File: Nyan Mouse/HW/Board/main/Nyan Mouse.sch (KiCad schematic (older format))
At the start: 11 parts, among them M101 BATTBALANCE-2S, P101 CONN_20X2, P102 CONN_4, P103 CONN_2, P104 CONN_2, U101 DRV8837, U102 DRV8837

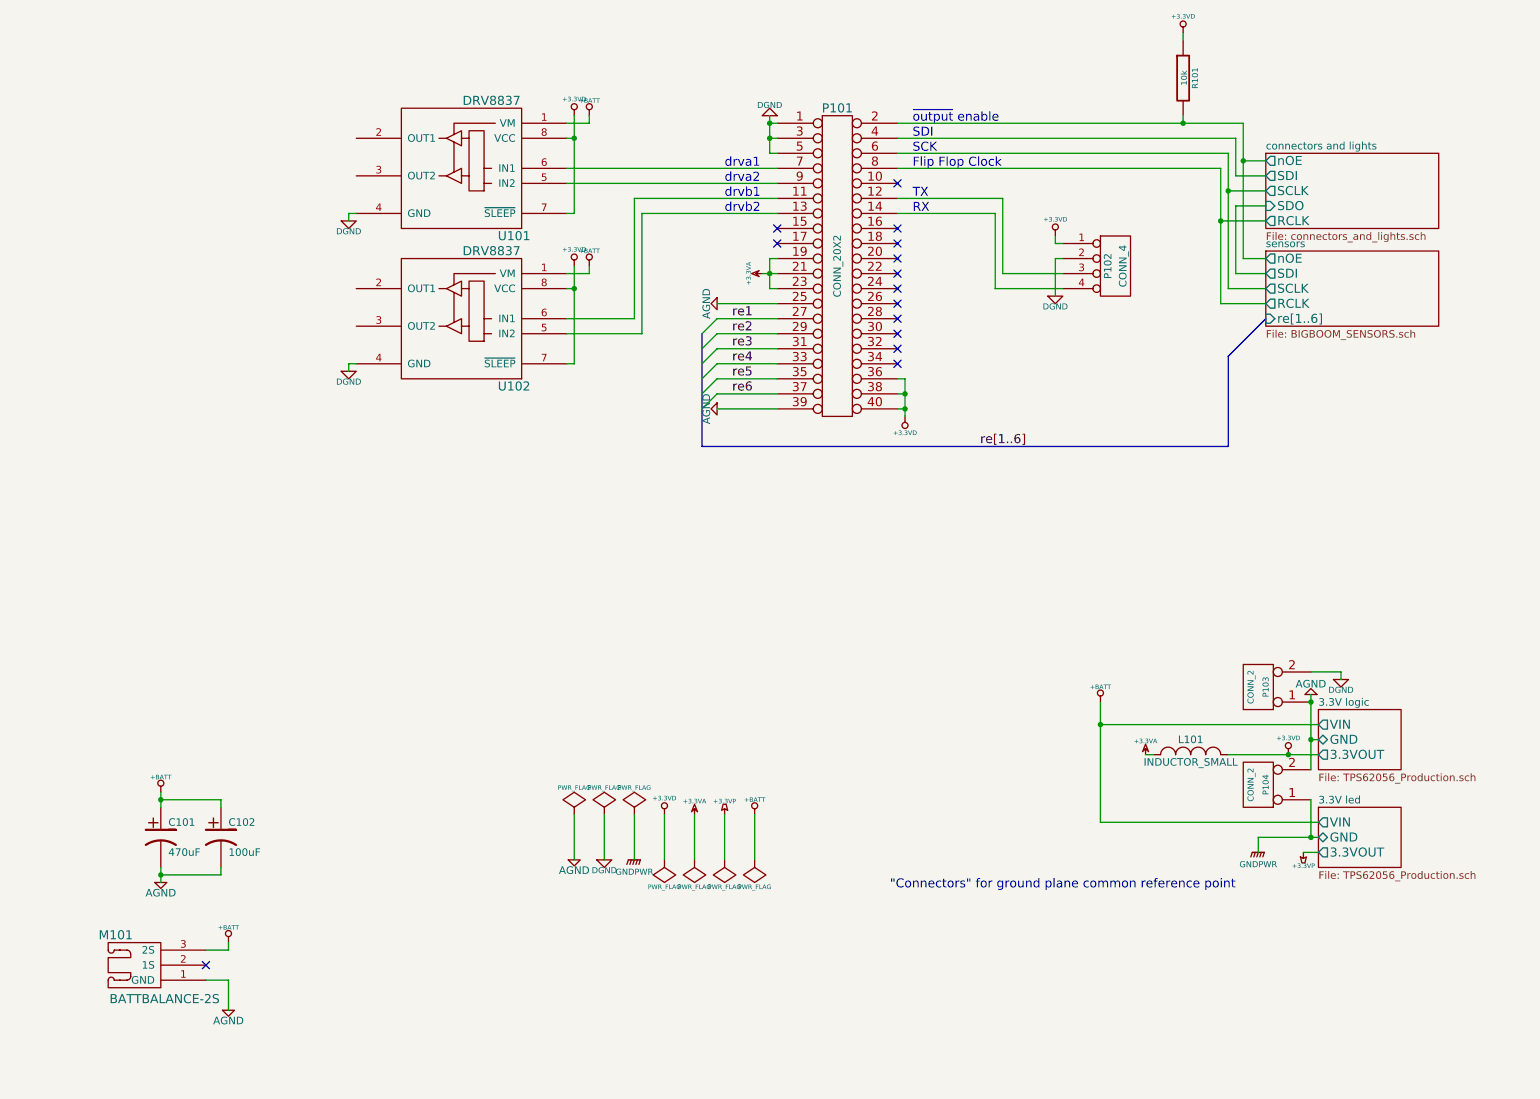
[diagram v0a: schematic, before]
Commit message: Finalized connector structure.
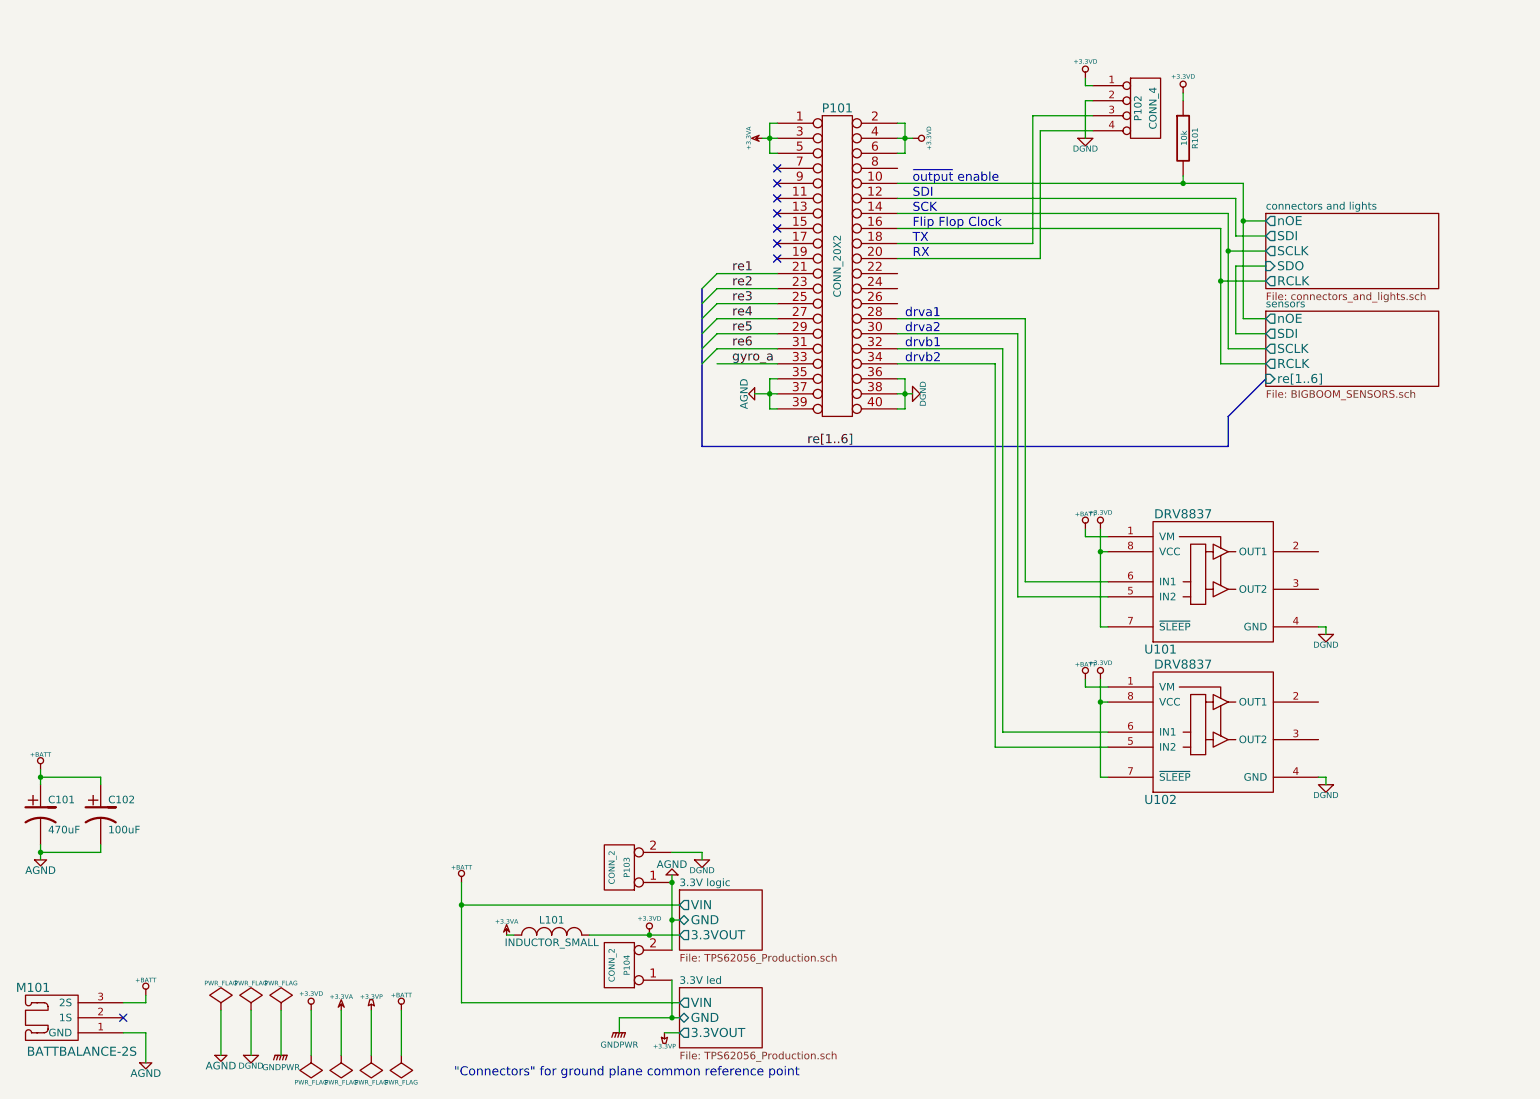
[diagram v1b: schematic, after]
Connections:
- net +3.3VA: now also P101.1 (P1), P101.3 (P3), P101.5 (P5); no longer P101.19 (P19), P101.21 (P21), P101.23 (P23)
- net +3.3VD: now also P101.2 (P2), P101.4 (P4), P101.6 (P6); no longer P101.36 (P36), P101.38 (P38), P101.40 (P40)
- net AGND: now also P101.35 (P35), P101.37 (P37); no longer P101.25
- net DGND: now also P101.36 (P36), P101.38 (P38), P101.40 (P40); no longer P101.1 (P1), P101.3 (P3), P101.5 (P5)
- net connectors and lights/RCLK: now also P101.16 (P16); no longer P101.8 (P8)
- net connectors and lights/SCLK: now also P101.14 (P14); no longer P101.6 (P6)
- net connectors and lights/SDI: now also P101.12 (P12); no longer P101.4 (P4)
- net connectors and lights/nOE: now also P101.10 (P10); no longer P101.2 (P2)
- net re1: now also P101.21 (P21); no longer P101.27 (P27)
- net re2: now also P101.23 (P23); no longer P101.29 (P29)
- net re3: now also P101.25; no longer P101.31 (P31)
- net re4: now also P101.27 (P27); no longer P101.33 (P33)
- net re5: now also P101.29 (P29); no longer P101.35 (P35)
- net re6: now also P101.31 (P31); no longer P101.37 (P37)
- net at P101.11 (P11): no longer U102.6 (IN1)
- net at P102.3 (P3): now also P101.18 (P18); no longer P101.12 (P12)
- net at P101.13 (P13): no longer U102.5 (IN2)
- net at P102.4 (P4): now also P101.20 (P20); no longer P101.14 (P14)
- net at P101.28 (P28): now also U101.6 (IN1)
- net at P101.30 (P30): now also U101.5 (IN2)
- net at P101.32 (P32): now also U102.6 (IN1)
- net at P101.34 (P34): now also U102.5 (IN2)
- net at P101.7 (P7): no longer U101.6 (IN1)
- net at P101.9 (P9): no longer U101.5 (IN2)
- new net gyro_a: P101.33 (P33)
- no-connect marks 14 -> 8
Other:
- moved on the sheet: C101, C102, L101, M101, P102, P103, P104, R101, U101, U102
